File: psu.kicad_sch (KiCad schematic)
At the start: 7 parts, among them Q6 BSS84, SW1 SW_SPDT, U2 AP7380-33Y-13

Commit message: grigila
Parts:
- SW1: footprint (none) -> digikey-footprints:Switch_Slide_JS202011SCQN

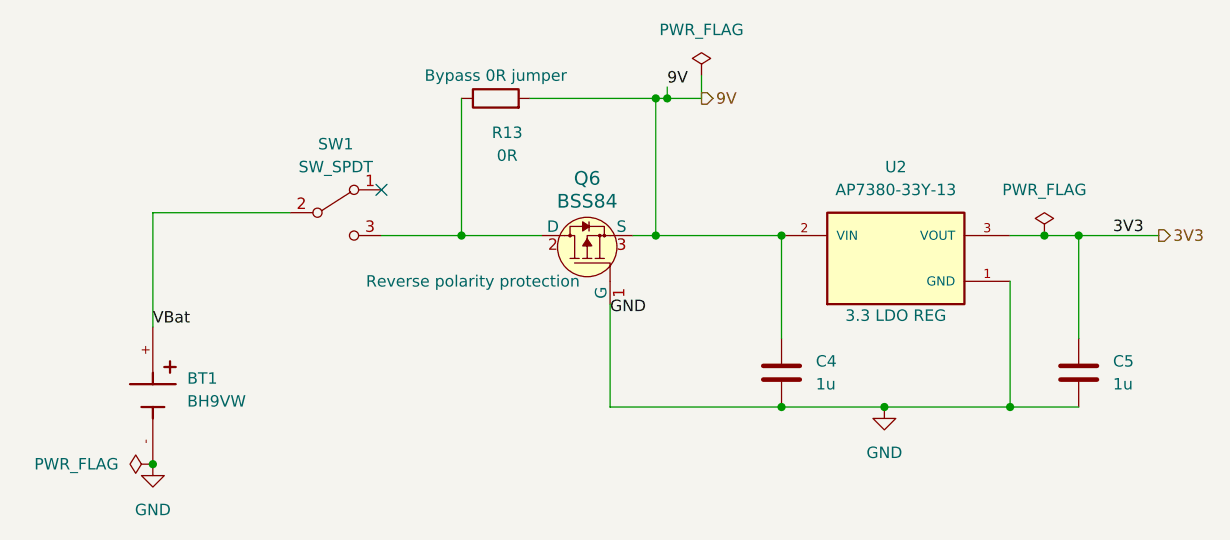
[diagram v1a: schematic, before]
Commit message: nuovo regolatore
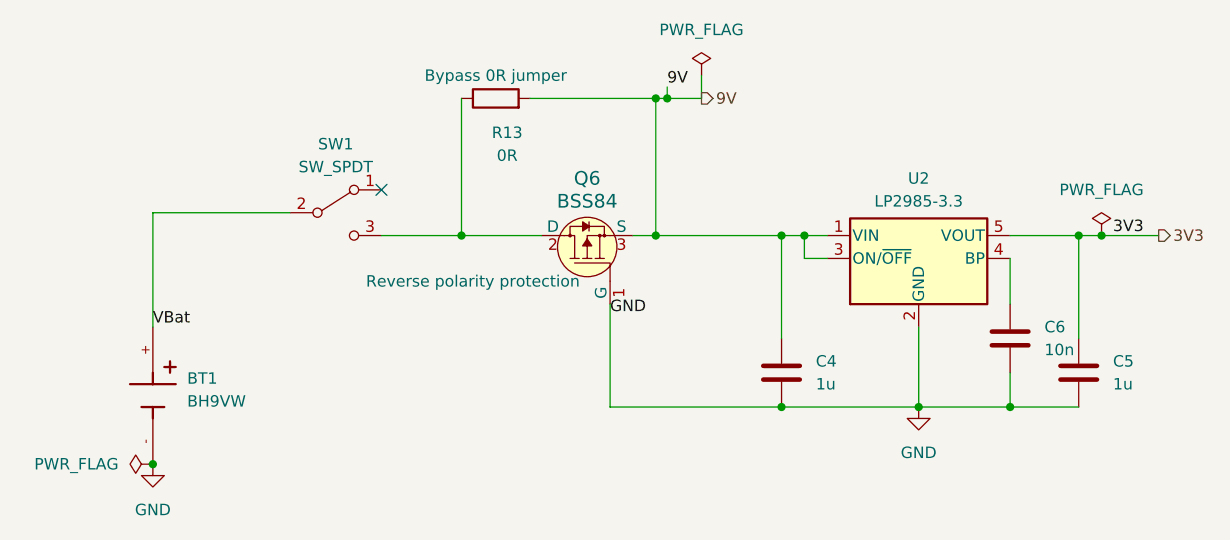
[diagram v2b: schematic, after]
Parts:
- removed U2: AP7380-33Y-13, AP7380-33Y-13:VREG_AP7380-33Y-13, symbol AP7380-33Y-13:AP7380-33Y-13
- added C6: 10n, Capacitor_SMD:C_0805_2012Metric, symbol Device:C
- added U2: LP2985-3.3, Package_TO_SOT_SMD:SOT-23-5, symbol Regulator_Linear:LP2985-3.3
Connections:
- net 3V3: now also U2.5 (VOUT)
- net 9V: now also U2.1 (VIN), U2.3 (ON/~{OFF})
- net GND: now also C6.2, U2.2 (GND)
- new net: C6.1, U2.4 (BP)
